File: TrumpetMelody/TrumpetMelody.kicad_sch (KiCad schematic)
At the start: 79 parts, among them J1 USB_B_Micro, J2 Conn_01x05, SW1 SW_Push, SW2 SW_SPST, SW3 SW_SPST, SW4 SW_SPST, U1 STM32F411RETx, U2 TLV62565DBVR, U3 MAX98357AETE+T, Y1 8MHz

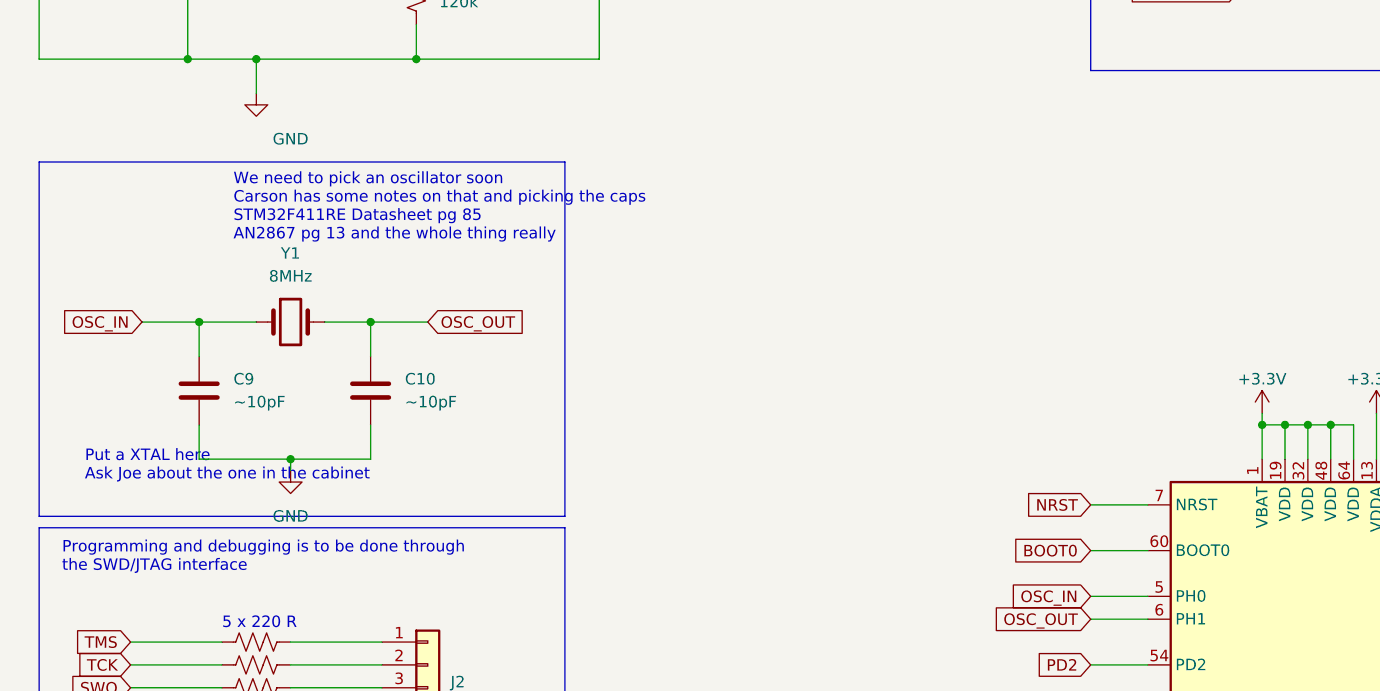
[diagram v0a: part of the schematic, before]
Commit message: test
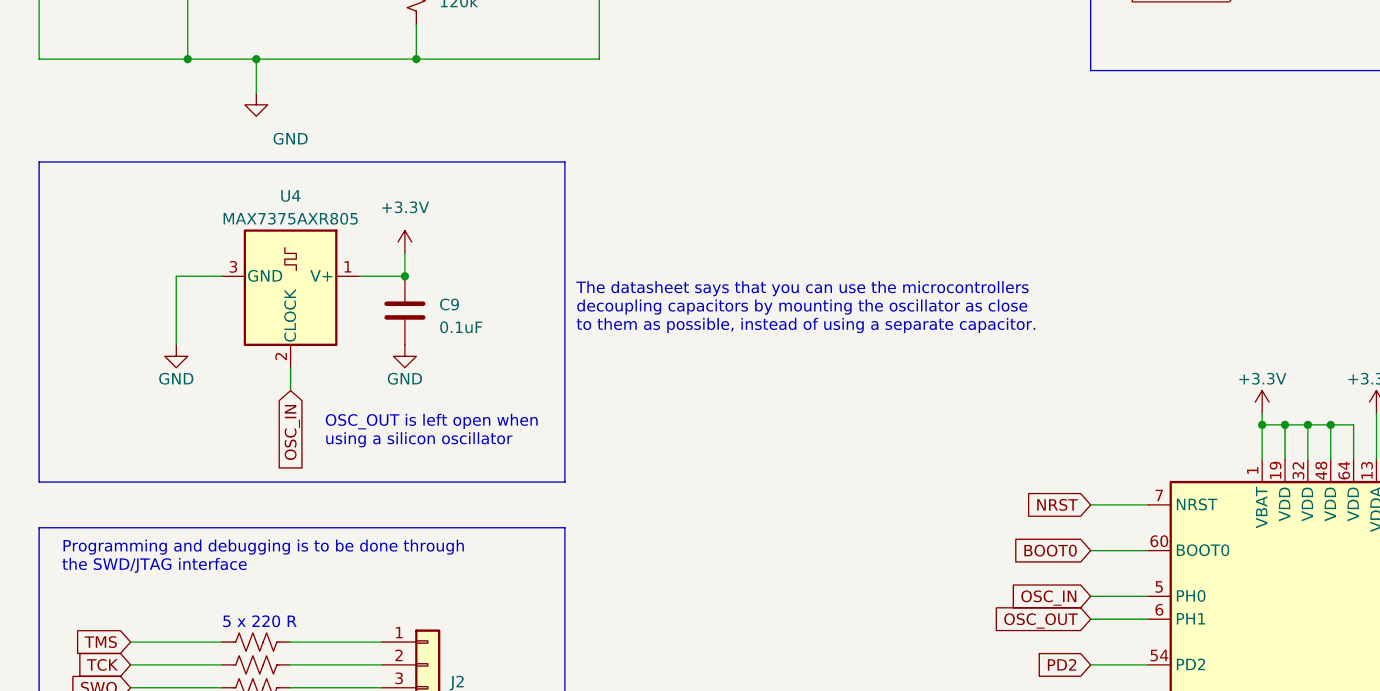
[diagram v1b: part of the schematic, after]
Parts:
- removed C10: ~10pF, symbol Device:C
- removed Y1: 8MHz, symbol Device:Crystal
- added U4: MAX7375AXR805, Package_TO_SOT_SMD:SOT-323_SC-70, symbol Oscillator:MAX7375AXR805
- C9: value ~10pF -> 0.1uF; footprint (none) -> Capacitor_SMD:C_0805_2012Metric_Pad1.18x1.45mm_HandSolder
- J2: footprint (none) -> Connector_PinHeader_2.54mm:PinHeader_1x05_P2.54mm_Vertical
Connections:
- net +3.3V: now also C9.1, U4.1 (V+)
- net GND: now also U4.3 (GND)
- net OSC_IN: now also U4.2 (CLOCK); no longer C9.1
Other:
- note added: "OSC_OUT is left open when using a silicon oscillator"
- note added: "The datasheet says that you can use the microcontrollers decoupling capacitors by mounting the oscillator as close to them as possible, instead of using a separate capacitor."
- note removed: "Put a XTAL here Ask Joe about the one in the cabinet"
- note removed: "We need to pick an oscillator soon Carson has some notes on that and picking the caps STM32F411RE Datasheet pg 85 AN2867 pg 13 and the whole thing really"
